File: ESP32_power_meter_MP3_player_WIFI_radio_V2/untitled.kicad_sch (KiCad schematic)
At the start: 40 parts, among them IC2 INA2181A4QDGSRQ1, J10 Conn_01x02, J11 USB_A, J12 Conn_01x03, J5 Barrel_Jack_Switch, J6 Conn_01x02, J7 Barrel_Jack_Switch, J8 USB_A, J9 Conn_01x03, U6 LM324

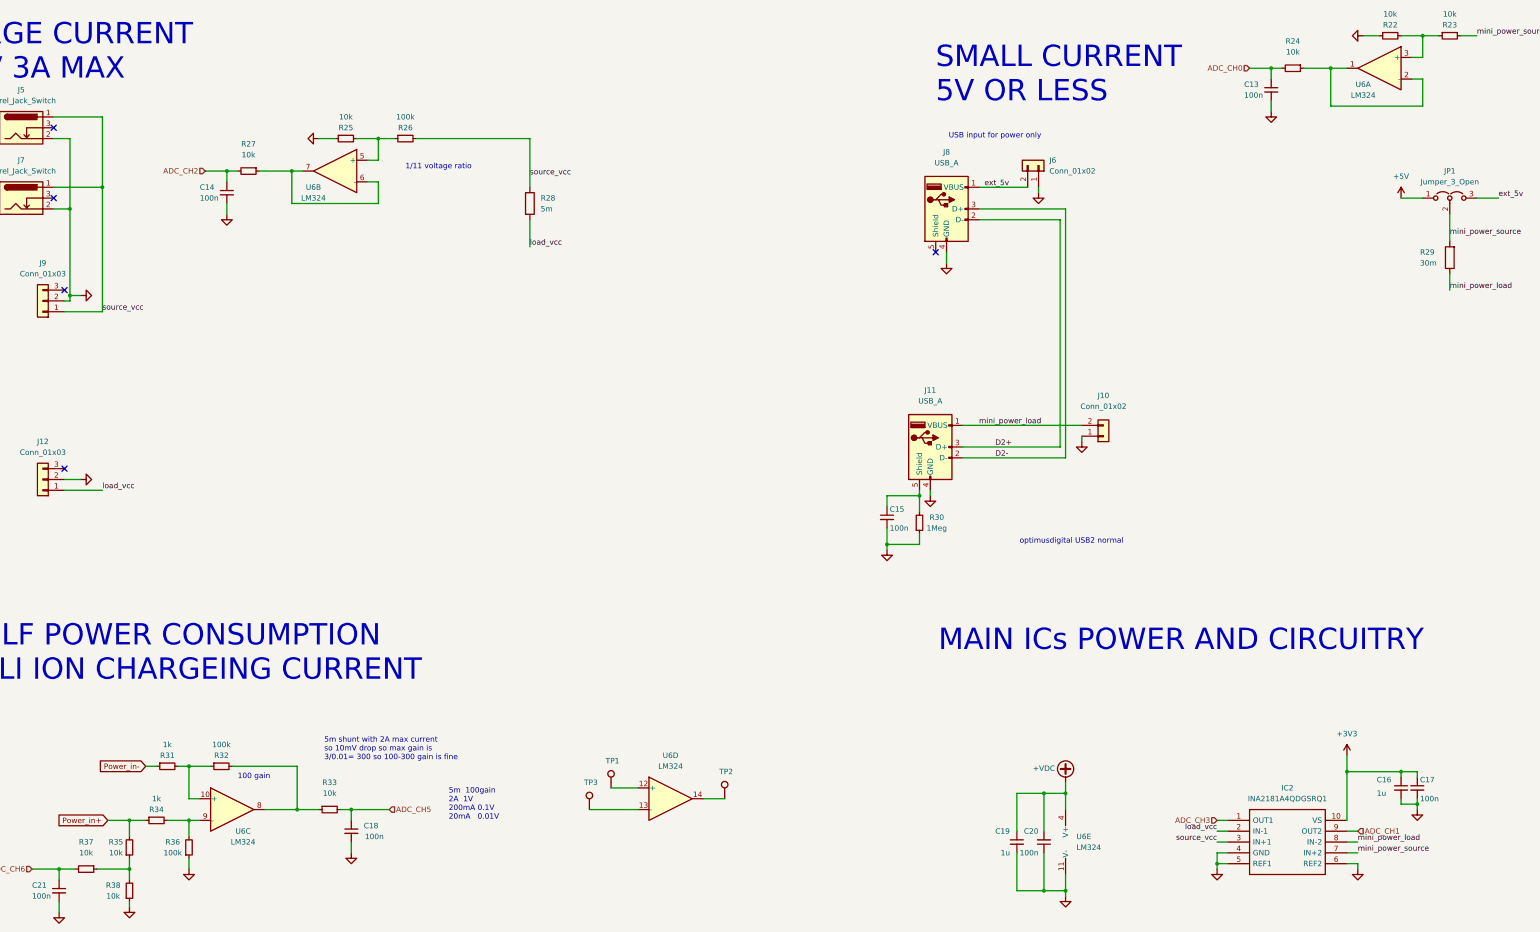
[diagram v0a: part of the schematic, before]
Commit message: f
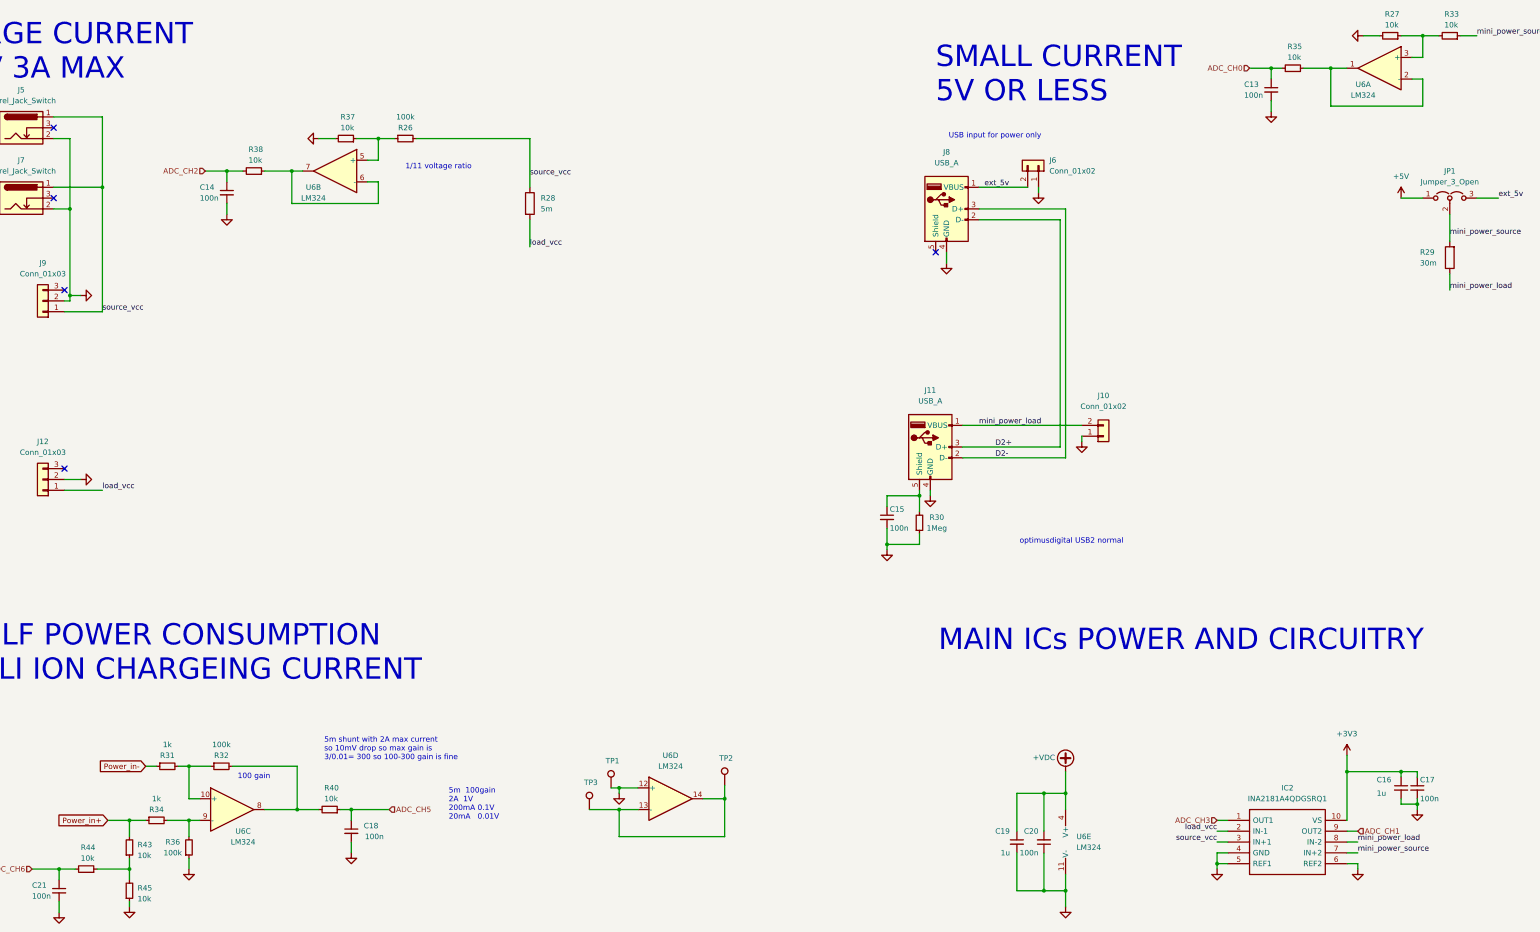
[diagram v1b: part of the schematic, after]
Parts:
- removed R22, R23, R24, R25: 10k, Resistor_SMD:R_0603_1608Metric_Pad0.98x0.95mm_HandSolder, symbol Device:R_Small
- added R40, R43, R44, R45: 10k, Resistor_SMD:R_0603_1608Metric, symbol Device:R_Small
- R27, R33, R35, R37, R38: footprint Resistor_SMD:R_0603_1608Metric_Pad0.98x0.95mm_HandSolder -> Resistor_SMD:R_0603_1608Metric; LCSC (none) -> C25804
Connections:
- net ADC_CH0: now also R35.2
- net ADC_CH2: now also R38.2; no longer R27.2
- net ADC_CH5: now also R40.1; no longer R33.2
- net ADC_CH6: now also R44.2; no longer R37.2
- net GND: now also R27.2, R37.2, TP1.1, U6.12 (+), R45.1; no longer R38.1
- net Power_in+: now also R43.2; no longer R35.2
- net mini_power_source: now also R33.1
- net at U6.3 (+): now also R27.1, R33.2
- net at R32.2, U6.8: now also R40.2; no longer R33.1
- net at R26.1, U6.5 (+): now also R37.1
- net at TP3.1, U6.13 (-): now also TP2.1, U6.14
- net at U6.1, U6.2 (-): now also R35.1
- net at U6.6 (-), U6.7: now also R38.1; no longer R27.1
- new net: R43.1, R44.1, R45.2
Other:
- moved on the sheet: TP2

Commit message: n
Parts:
- C13: LCSCC (none) -> C14663
- C14, C15, C18, C21: LCSC (none) -> C14663
- C16, C17, C20: LCSC (none) -> C1623
- R31, R34: LCSC (none) -> C21190
- R32, R36: LCSC (none) -> C25803
- U6: footprint (none) -> Package_SO:SOIC-14_3.9x8.7mm_P1.27mm; LCSC (none) -> C71035
- U6: LCSC (none) -> C71035
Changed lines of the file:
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@@
+      (effects (font (size 1.27 1.27)) hide)
+    )
+    (property "LCSC" "C25803" (id 4) (at 82.55 214.63 0)
       (effects (font (size 1.27 1.27)) hide)
     )
@@
       (effects (font (size 1.27 1.27)) hide)
     )
+    (property "LCSC" "C1623" (id 4) (at 367.03 200.66 0)
+      (effects (font (size 1.27 1.27)) hide)
+    )
     (pin "1")
     (pin "2")
@@
     (property "Reference" "U6" (id 0) (at 95.25 210.82 0))
     (property "Value" "LM324" (id 1) (at 95.25 213.36 0))
-    (property "Footprint" "" (id 2) (at 91.44 203.2 0)
+    (property "Footprint" "Package_SO:SOIC-14_3.9x8.7mm_P1.27mm" (id 2) (at 91.44 203.2 0)
       (effects (font (size 1.27 1.27)) hide)
     )
     (property "Datasheet" "http://www.ti.com/lit/ds/symlink/lm2902-n.pdf" (id 3) (at 93.98 200.66 0)
+      (effects (font (size 1.27 1.27)) hide)
+    )
+    (property "LCSC" "C71035" (id 4) (at 92.71 205.74 0)
       (effects (font (size 1.27 1.27)) hide)
     )
@@
       (effects (font (size 1.27 1.27)) hide)
     )
+    (property "LCSC" "C14663" (id 4) (at 52.07 224.79 0)
+      (effects (font (size 1.27 1.27)) hide)
+    )
     (pin "1")
     (pin "2")
@@
     )
     (property "Datasheet" "~" (id 3) (at 246.38 137.16 0)
+      (effects (font (size 1.27 1.27)) hide)
+    )
+    (property "LCSC" "C14663" (id 4) (at 246.38 137.16 0)
       (effects (font (size 1.27 1.27)) hide)
     )
@@
       (effects (font (size 1.27 1.27)) hide)
     )
+    (property "LCSC" "C1623" (id 4) (at 283.21 213.36 0)
+      (effects (font (size 1.27 1.27)) hide)
+    )
     (pin "1")
     (pin "2")
@@
       (effects (font (size 1.27 1.27)) hide)
     )
+    (property "LCSC" "C1623" (id 4) (at 370.84 200.66 0)
+      (effects (font (size 1.27 1.27)) hide)
+    )
     (pin "1")
     (pin "2")
@@
     (property "Reference" "U6" (id 0) (at 358.14 35.56 0))
     (property "Value" "LM324" (id 1) (at 358.14 38.1 0))
-    (property "Footprint" "" (id 2) (at 363.22 29.21 0)
+    (property "Footprint" "Package_SO:SOIC-14_3.9x8.7mm_P1.27mm" (id 2) (at 363.22 29.21 0)
       (effects (font (size 1.27 1.27)) hide)
     )
     (property "Datasheet" "http://www.ti.com/lit/ds/symlink/lm2902-n.pdf" (id 3) (at 360.68 26.67 0)
+      (effects (font (size 1.27 1.27)) hide)
+    )
+    (property "LCSC" "C71035" (id 4) (at 361.95 31.75 0)
       (effects (font (size 1.27 1.27)) hide)
     )
@@
       (effects (font (size 1.27 1.27)) hide)
     )
+    (property "LCSC" "C14663" (id 4) (at 120.65 210.82 0)
+      (effects (font (size 1.27 1.27)) hide)
+    )
     (pin "1")
     (pin "2")
@@
       (effects (font (size 1.27 1.27)) hide)
     )
+    (property "LCSC" "C21190" (id 4) (at 77.47 195.58 90)
+      (effects (font (size 1.27 1.27)) hide)
+    )
     (pin "1")
     (pin "2")
@@
       (effects (font (size 1.27 1.27)) hide)
     )
+    (property "LCSC" "C21190" (id 4) (at 74.93 208.28 90)
+      (effects (font (size 1.27 1.27)) hide)
+    )
     (pin "1")
     (pin "2")
@@
       (effects (font (size 1.27 1.27)) (justify left))
     )
-    (property "Footprint" "" (id 2) (at 289.56 210.82 0)
+    (property "Footprint" "Package_SO:SOIC-14_3.9x8.7mm_P1.27mm" (id 2) (at 289.56 210.82 0)
       (effects (font (size 1.27 1.27)) hide)
     )
     (property "Datasheet" "http://www.ti.com/lit/ds/symlink/lm2902-n.pdf" (id 3) (at 292.1 208.28 0)
+      (effects (font (size 1.27 1.27)) hide)
+    )
+    (property "LCSC" "C71035" (id 4) (at 290.83 213.36 0)
       (effects (font (size 1.27 1.27)) hide)
     )
@@
     (property "Reference" "U6" (id 0) (at 111.76 59.69 0))
     (property "Value" "LM324" (id 1) (at 111.76 62.23 0))
-    (property "Footprint" "" (id 2) (at 118.11 53.34 0)
+    (property "Footprint" "Package_SO:SOIC-14_3.9x8.7mm_P1.27mm" (id 2) (at 118.11 53.34 0)
       (effects (font (size 1.27 1.27)) hide)
     )
     (property "Datasheet" "http://www.ti.com/lit/ds/symlink/lm2902-n.pdf" (id 3) (at 115.57 50.8 0)
+      (effects (font (size 1.27 1.27)) hide)
+    )
+    (property "LCSC" "C71035" (id 4) (at 116.84 55.88 0)
       (effects (font (size 1.27 1.27)) hide)
     )
@@
       (effects (font (size 1.27 1.27)) hide)
     )
+    (property "LCSC" "C25803" (id 4) (at 90.17 195.58 90)
+      (effects (font (size 1.27 1.27)) hide)
+    )
     (pin "1")
     (pin "2")
@@
     )
     (property "Datasheet" "http://www.ti.com/lit/ds/symlink/lm2902-n.pdf" (id 3) (at 196.85 198.12 0)
+      (effects (font (size 1.27 1.27)) hide)
+    )
+    (property "LCSC" "C71035" (id 4) (at 195.58 203.2 0)
       (effects (font (size 1.27 1.27)) hide)
     )
@@
       (effects (font (size 1.27 1.27)) hide)
     )
+    (property "LCSC" "C14663" (id 4) (at 91.44 60.96 0)
+      (effects (font (size 1.27 1.27)) hide)
+    )
     (pin "1")
     (pin "2")
@@
       (effects (font (size 1.27 1.27)) hide)
     )
+    (property "LCSCC" "C14663" (id 4) (at 336.55 36.83 0)
+      (effects (font (size 1.27 1.27)) hide)
+    )
